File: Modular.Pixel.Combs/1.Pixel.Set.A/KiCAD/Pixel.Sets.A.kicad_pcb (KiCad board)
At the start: 2 copper layers, 78 x 78 mm, 19 parts

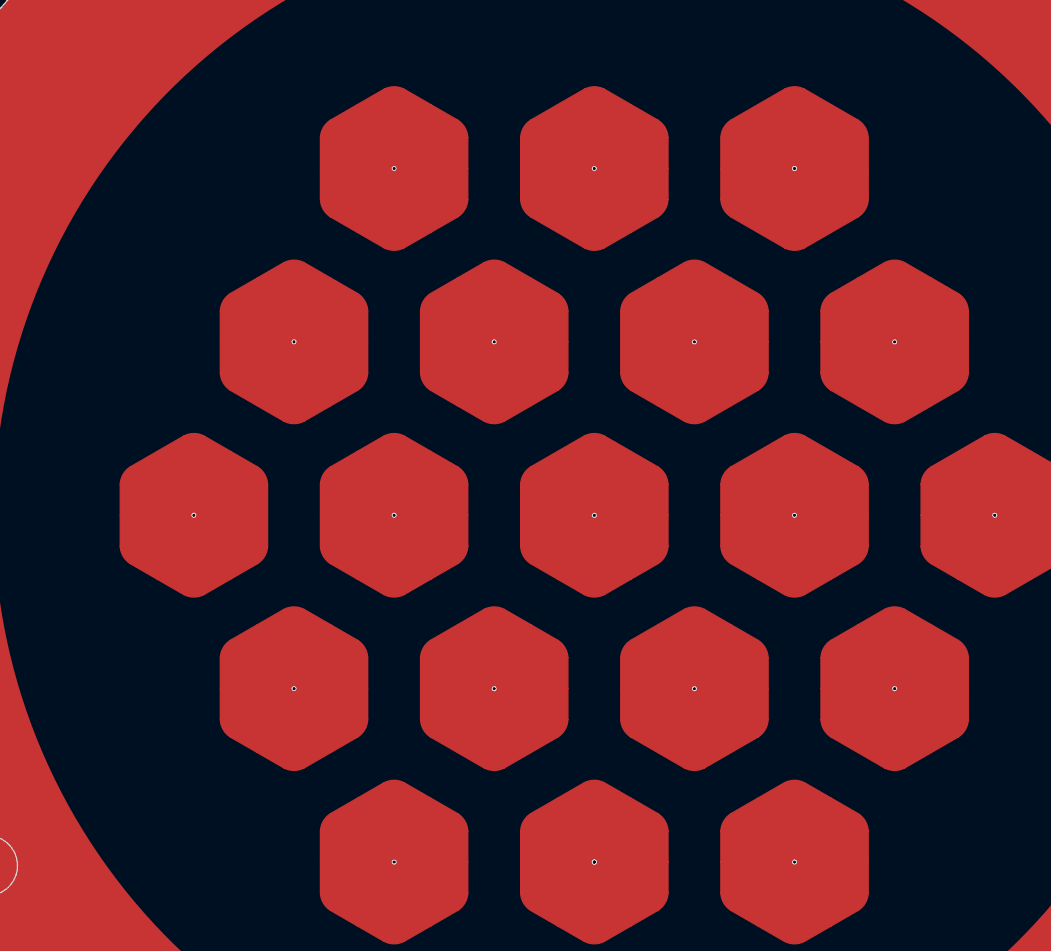
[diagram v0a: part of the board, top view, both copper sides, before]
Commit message: Finalized Pixel Plane Design
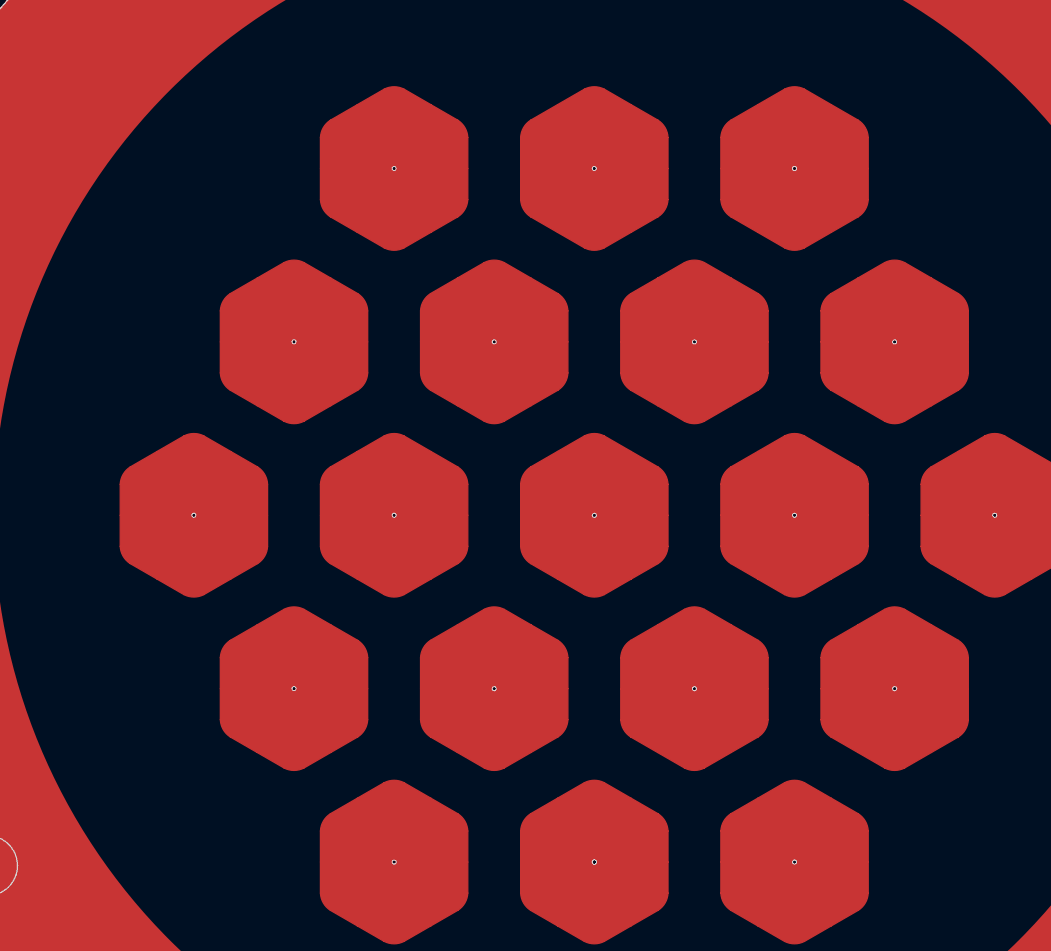
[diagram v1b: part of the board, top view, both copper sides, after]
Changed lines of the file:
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@@
     (fp_arc (start -1.549999 3.68) (mid -2.041539 3.53605) (end -2.411974 3.182339)
       (stroke (width 0.01) (type default)) (layer "F.Cu"))
-    (fp_arc (start 1.549999 -3.68) (mid 2.041539 -3.536049) (end 2.411974 -3.182339)
+    (fp_arc (start 1.549999 -3.68) (mid 2.04154 -3.53605) (end 2.411974 -3.182339)
       (stroke (width 0.01) (type default)) (layer "F.Cu"))
     (fp_arc (start 2.411974 3.182339) (mid 2.04154 3.536051) (end 1.549999 3.68)
@@
     (fp_arc (start -1.549999 3.68) (mid -2.041539 3.53605) (end -2.411974 3.182339)
       (stroke (width 0.01) (type default)) (layer "F.Cu"))
-    (fp_arc (start 1.549999 -3.68) (mid 2.041539 -3.536049) (end 2.411974 -3.182339)
+    (fp_arc (start 1.549999 -3.68) (mid 2.04154 -3.53605) (end 2.411974 -3.182339)
       (stroke (width 0.01) (type default)) (layer "F.Cu"))
     (fp_arc (start 2.411974 3.182339) (mid 2.04154 3.536051) (end 1.549999 3.68)
@@
     (fp_arc (start -1.549999 3.68) (mid -2.041539 3.53605) (end -2.411974 3.182339)
       (stroke (width 0.01) (type default)) (layer "F.Cu"))
-    (fp_arc (start 1.549999 -3.68) (mid 2.041539 -3.536049) (end 2.411974 -3.182339)
+    (fp_arc (start 1.549999 -3.68) (mid 2.04154 -3.53605) (end 2.411974 -3.182339)
       (stroke (width 0.01) (type default)) (layer "F.Cu"))
     (fp_arc (start 2.411974 3.182339) (mid 2.04154 3.536051) (end 1.549999 3.68)
@@
     (fp_arc (start -1.549999 3.68) (mid -2.041539 3.53605) (end -2.411974 3.182339)
       (stroke (width 0.01) (type default)) (layer "F.Cu"))
-    (fp_arc (start 1.549999 -3.68) (mid 2.041539 -3.536049) (end 2.411974 -3.182339)
+    (fp_arc (start 1.549999 -3.68) (mid 2.04154 -3.53605) (end 2.411974 -3.182339)
       (stroke (width 0.01) (type default)) (layer "F.Cu"))
     (fp_arc (start 2.411974 3.182339) (mid 2.04154 3.536051) (end 1.549999 3.68)
@@
     (fp_arc (start -1.549999 3.68) (mid -2.041539 3.53605) (end -2.411974 3.182339)
       (stroke (width 0.01) (type default)) (layer "F.Cu"))
-    (fp_arc (start 1.549999 -3.68) (mid 2.041539 -3.536049) (end 2.411974 -3.182339)
+    (fp_arc (start 1.549999 -3.68) (mid 2.04154 -3.53605) (end 2.411974 -3.182339)
       (stroke (width 0.01) (type default)) (layer "F.Cu"))
     (fp_arc (start 2.411974 3.182339) (mid 2.04154 3.536051) (end 1.549999 3.68)
@@
     (fp_arc (start -1.549999 3.68) (mid -2.041539 3.53605) (end -2.411974 3.182339)
       (stroke (width 0.01) (type default)) (layer "F.Cu"))
-    (fp_arc (start 1.549999 -3.68) (mid 2.041539 -3.536049) (end 2.411974 -3.182339)
+    (fp_arc (start 1.549999 -3.68) (mid 2.04154 -3.53605) (end 2.411974 -3.182339)
       (stroke (width 0.01) (type default)) (layer "F.Cu"))
     (fp_arc (start 2.411974 3.182339) (mid 2.04154 3.536051) (end 1.549999 3.68)
@@
     (fp_arc (start -1.549999 3.68) (mid -2.041539 3.53605) (end -2.411974 3.182339)
       (stroke (width 0.01) (type default)) (layer "F.Cu"))
-    (fp_arc (start 1.549999 -3.68) (mid 2.041539 -3.536049) (end 2.411974 -3.182339)
+    (fp_arc (start 1.549999 -3.68) (mid 2.04154 -3.53605) (end 2.411974 -3.182339)
       (stroke (width 0.01) (type default)) (layer "F.Cu"))
     (fp_arc (start 2.411974 3.182339) (mid 2.04154 3.536051) (end 1.549999 3.68)
@@
     (fp_arc (start -1.549999 3.68) (mid -2.041539 3.53605) (end -2.411974 3.182339)
       (stroke (width 0.01) (type default)) (layer "F.Cu"))
-    (fp_arc (start 1.549999 -3.68) (mid 2.041536 -3.536048) (end 2.411974 -3.182339)
+    (fp_arc (start 1.549999 -3.68) (mid 2.041539 -3.536049) (end 2.411974 -3.182339)
       (stroke (width 0.01) (type default)) (layer "F.Cu"))
     (fp_arc (start 2.411974 3.182339) (mid 2.04154 3.536051) (end 1.549999 3.68)
@@
     (fp_arc (start -1.549999 3.68) (mid -2.041539 3.53605) (end -2.411974 3.182339)
       (stroke (width 0.01) (type default)) (layer "F.Cu"))
-    (fp_arc (start 1.549999 -3.68) (mid 2.041539 -3.536049) (end 2.411974 -3.182339)
+    (fp_arc (start 1.549999 -3.68) (mid 2.04154 -3.53605) (end 2.411974 -3.182339)
       (stroke (width 0.01) (type default)) (layer "F.Cu"))
     (fp_arc (start 2.411974 3.182339) (mid 2.04154 3.536051) (end 1.549999 3.68)
@@
     (fp_arc (start -1.549999 3.68) (mid -2.041539 3.53605) (end -2.411974 3.182339)
       (stroke (width 0.01) (type default)) (layer "F.Cu"))
-    (fp_arc (start 1.549999 -3.68) (mid 2.041539 -3.536049) (end 2.411974 -3.182339)
+    (fp_arc (start 1.549999 -3.68) (mid 2.04154 -3.53605) (end 2.411974 -3.182339)
       (stroke (width 0.01) (type default)) (layer "F.Cu"))
     (fp_arc (start 2.411974 3.182339) (mid 2.04154 3.536051) (end 1.549999 3.68)
@@
     (fp_arc (start -1.549999 3.68) (mid -2.041539 3.53605) (end -2.411974 3.182339)
       (stroke (width 0.01) (type default)) (layer "F.Cu"))
-    (fp_arc (start 1.549999 -3.68) (mid 2.041539 -3.536049) (end 2.411974 -3.182339)
+    (fp_arc (start 1.549999 -3.68) (mid 2.04154 -3.53605) (end 2.411974 -3.182339)
       (stroke (width 0.01) (type default)) (layer "F.Cu"))
     (fp_arc (start 2.411974 3.182339) (mid 2.04154 3.536051) (end 1.549999 3.68)
@@
     (fp_arc (start -1.549999 3.68) (mid -2.041539 3.53605) (end -2.411974 3.182339)
       (stroke (width 0.01) (type default)) (layer "F.Cu"))
-    (fp_arc (start 1.549999 -3.68) (mid 2.041539 -3.536049) (end 2.411974 -3.182339)
+    (fp_arc (start 1.549999 -3.68) (mid 2.04154 -3.53605) (end 2.411974 -3.182339)
       (stroke (width 0.01) (type default)) (layer "F.Cu"))
     (fp_arc (start 2.411974 3.182339) (mid 2.04154 3.536051) (end 1.549999 3.68)
@@
     (fp_arc (start -1.549999 3.68) (mid -2.041539 3.53605) (end -2.411974 3.182339)
       (stroke (width 0.01) (type default)) (layer "F.Cu"))
-    (fp_arc (start 1.549999 -3.68) (mid 2.041539 -3.536049) (end 2.411974 -3.182339)
+    (fp_arc (start 1.549999 -3.68) (mid 2.04154 -3.53605) (end 2.411974 -3.182339)
       (stroke (width 0.01) (type default)) (layer "F.Cu"))
     (fp_arc (start 2.411974 3.182339) (mid 2.04154 3.536051) (end 1.549999 3.68)
@@
     (fp_arc (start -1.549999 3.68) (mid -2.041539 3.53605) (end -2.411974 3.182339)
       (stroke (width 0.01) (type default)) (layer "F.Cu"))
-    (fp_arc (start 1.549999 -3.68) (mid 2.041539 -3.536049) (end 2.411974 -3.182339)
+    (fp_arc (start 1.549999 -3.68) (mid 2.04154 -3.53605) (end 2.411974 -3.182339)
       (stroke (width 0.01) (type default)) (layer "F.Cu"))
     (fp_arc (start 2.411974 3.182339) (mid 2.04154 3.536051) (end 1.549999 3.68)
@@
     (fp_arc (start -1.549999 3.68) (mid -2.041539 3.53605) (end -2.411974 3.182339)
       (stroke (width 0.01) (type default)) (layer "F.Cu"))
-    (fp_arc (start 1.549999 -3.68) (mid 2.041539 -3.536049) (end 2.411974 -3.182339)
+    (fp_arc (start 1.549999 -3.68) (mid 2.04154 -3.53605) (end 2.411974 -3.182339)
       (stroke (width 0.01) (type default)) (layer "F.Cu"))
     (fp_arc (start 2.411974 3.182339) (mid 2.04154 3.536051) (end 1.549999 3.68)
@@
     (fp_arc (start -1.549999 3.68) (mid -2.041539 3.53605) (end -2.411974 3.182339)
       (stroke (width 0.01) (type default)) (layer "F.Cu"))
-    (fp_arc (start 1.549999 -3.68) (mid 2.041539 -3.536049) (end 2.411974 -3.182339)
+    (fp_arc (start 1.549999 -3.68) (mid 2.04154 -3.53605) (end 2.411974 -3.182339)
       (stroke (width 0.01) (type default)) (layer "F.Cu"))
     (fp_arc (start 2.411974 3.182339) (mid 2.04154 3.536051) (end 1.549999 3.68)
@@
     (fp_arc (start -1.549999 3.68) (mid -2.041539 3.53605) (end -2.411974 3.182339)
       (stroke (width 0.01) (type default)) (layer "F.Cu"))
-    (fp_arc (start 1.549999 -3.68) (mid 2.041539 -3.536049) (end 2.411974 -3.182339)
+    (fp_arc (start 1.549999 -3.68) (mid 2.04154 -3.53605) (end 2.411974 -3.182339)
       (stroke (width 0.01) (type default)) (layer "F.Cu"))
     (fp_arc (start 2.411974 3.182339) (mid 2.04154 3.536051) (end 1.549999 3.68)
@@
     (fp_arc (start -1.549999 3.68) (mid -2.041539 3.53605) (end -2.411974 3.182339)
       (stroke (width 0.01) (type default)) (layer "F.Cu"))
-    (fp_arc (start 1.549999 -3.68) (mid 2.041539 -3.536049) (end 2.411974 -3.182339)
+    (fp_arc (start 1.549999 -3.68) (mid 2.04154 -3.53605) (end 2.411974 -3.182339)
       (stroke (width 0.01) (type default)) (layer "F.Cu"))
     (fp_arc (start 2.411974 3.182339) (mid 2.04154 3.536051) (end 1.549999 3.68)
@@
     (fp_arc (start -1.549999 3.68) (mid -2.041539 3.53605) (end -2.411974 3.182339)
       (stroke (width 0.01) (type default)) (layer "F.Cu"))
-    (fp_arc (start 1.549999 -3.68) (mid 2.041539 -3.536049) (end 2.411974 -3.182339)
+    (fp_arc (start 1.549999 -3.68) (mid 2.04154 -3.53605) (end 2.411974 -3.182339)
       (stroke (width 0.01) (type default)) (layer "F.Cu"))
     (fp_arc (start 2.411974 3.182339) (mid 2.04154 3.536051) (end 1.549999 3.68)
